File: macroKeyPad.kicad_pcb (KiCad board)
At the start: 2 copper layers, 17 parts, among them U1 kb2040

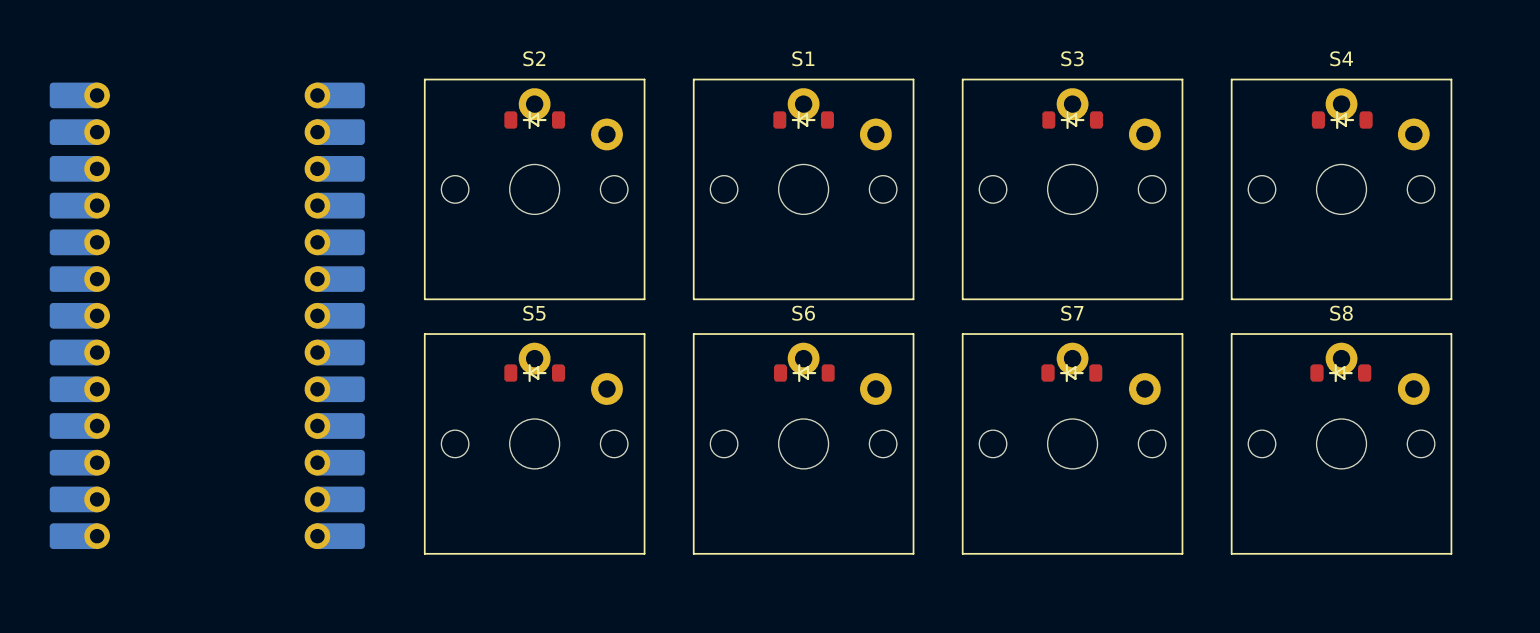
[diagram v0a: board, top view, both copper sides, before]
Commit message: pretty close to being done
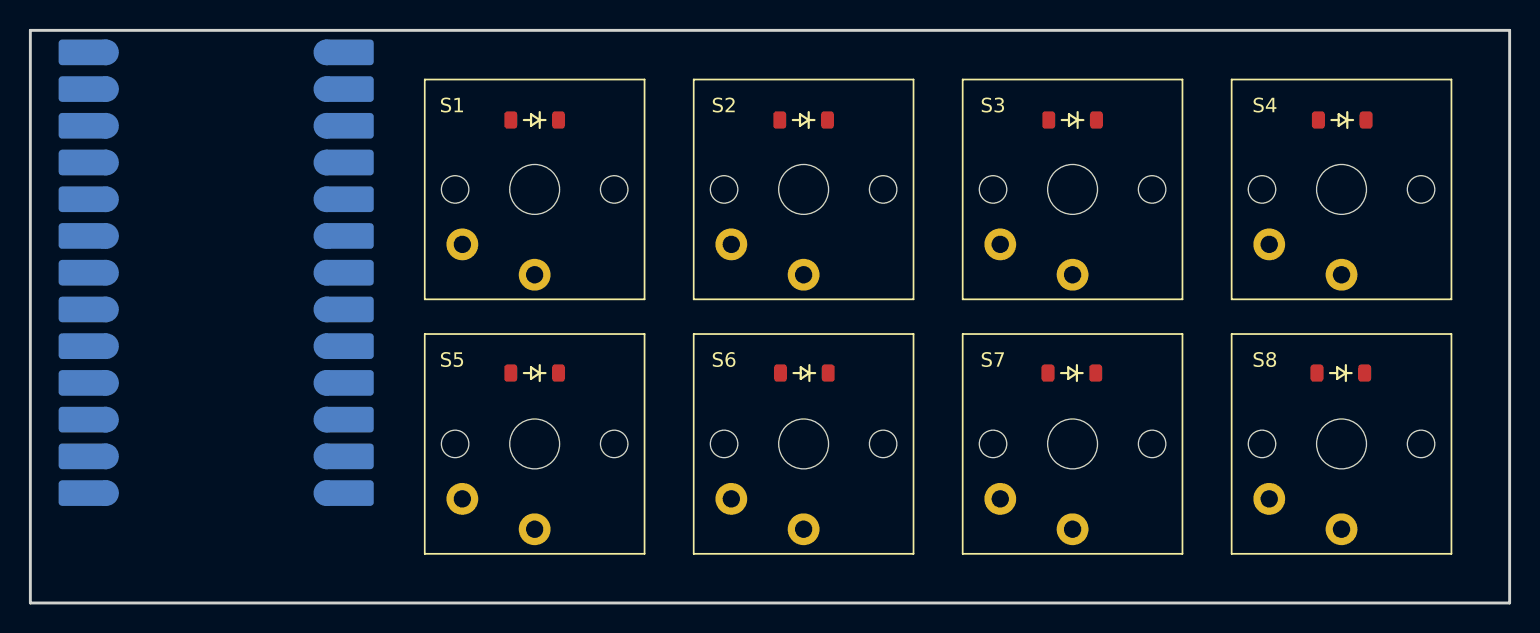
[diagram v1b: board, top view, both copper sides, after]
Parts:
- moved S1 18.6 mm to (98.5, 52.8), turned to 180 degrees
- moved S2 18.6 mm to (117.1, 52.8), turned to 180 degrees
- moved U1 3.04 mm to (76.5, 58.5)
- turned D1 to 180 degrees
- turned D2 to 180 degrees
- turned D3 to 180 degrees
- turned D4 to 180 degrees
- turned D5 to 180 degrees
- turned D6 to 180 degrees
- turned D7 to 180 degrees
- turned D8 to 180 degrees
- turned S3 to 180 degrees
- turned S4 to 180 degrees
- turned S5 to 180 degrees
- turned S6 to 180 degrees
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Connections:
- U1 pad 10: unconnected-(U1-D6-Pad10) -> Col1
- U1 pad 11: unconnected-(U1-D7-Pad11) -> Col0
- U1 pad 19: Col0 -> unconnected-(U1-A3/29-Pad19)
- U1 pad 20: Col1 -> unconnected-(U1-A2/28-Pad20)
- U1 pad 21: Col2 -> unconnected-(U1-A1/27-Pad21)
- U1 pad 22: Col3 -> unconnected-(U1-A0/26-Pad22)
- U1 pad 23: Row0 -> unconnected-(U1-SCK/18-Pad23)
- U1 pad 24: Row1 -> unconnected-(U1-MISO/20-Pad24)
- U1 pad 6: unconnected-(U1-D2-Pad6) -> Row1
- U1 pad 7: unconnected-(U1-D3-Pad7) -> Row0
- U1 pad 8: unconnected-(U1-D4-Pad8) -> Col3
- U1 pad 9: unconnected-(U1-D5-Pad9) -> Col2
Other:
- board outline added: 102.3 x 39.6 mm
